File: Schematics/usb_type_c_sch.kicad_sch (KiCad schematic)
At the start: 4 parts, among them J2 USB_C_Receptacle

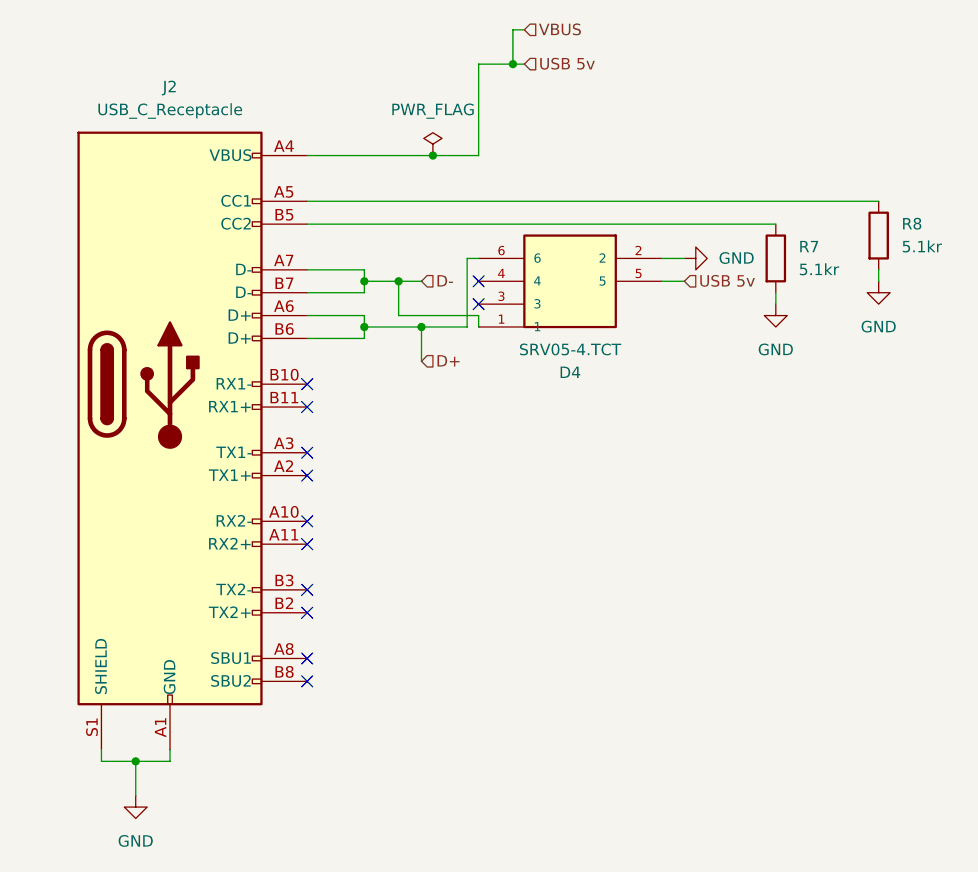
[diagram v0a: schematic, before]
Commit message: fixed schematic and named ready for bom to order
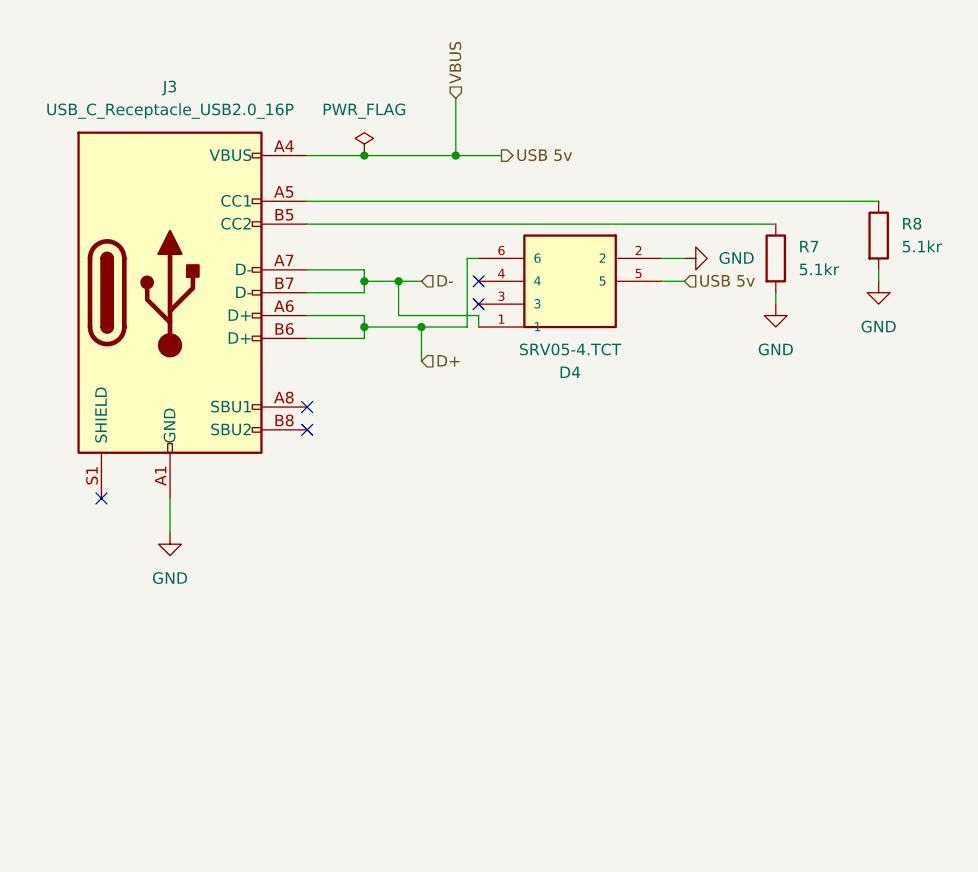
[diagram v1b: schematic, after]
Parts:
- removed J2: USB_C_Receptacle, Connector_USB:USB_C_Receptacle_HRO_TYPE-C-31-M-12, symbol Connector:USB_C_Receptacle
- added J3: USB_C_Receptacle_USB2.0_16P, Connector_USB:USB_C_Receptacle_HRO_TYPE-C-31-M-12, symbol Connector:USB_C_Receptacle_USB2.0_16P
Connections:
- net D+: now also J3.A6 (D+), J3.B6 (D+)
- net D-: now also J3.A7 (D-), J3.B7 (D-)
- net GND: now also J3.A1 (GND), J3.A12 (GND), J3.B1 (GND), J3.B12 (GND)
- net USB 5v: now also J3.A4 (VBUS), J3.A9 (VBUS), J3.B4 (VBUS), J3.B9 (VBUS)
- net at R8.1: now also J3.A5 (CC1)
- net at R7.1: now also J3.B5 (CC2)
- no-connect marks 12 -> 5
